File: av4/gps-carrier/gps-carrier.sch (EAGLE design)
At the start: 2 parts

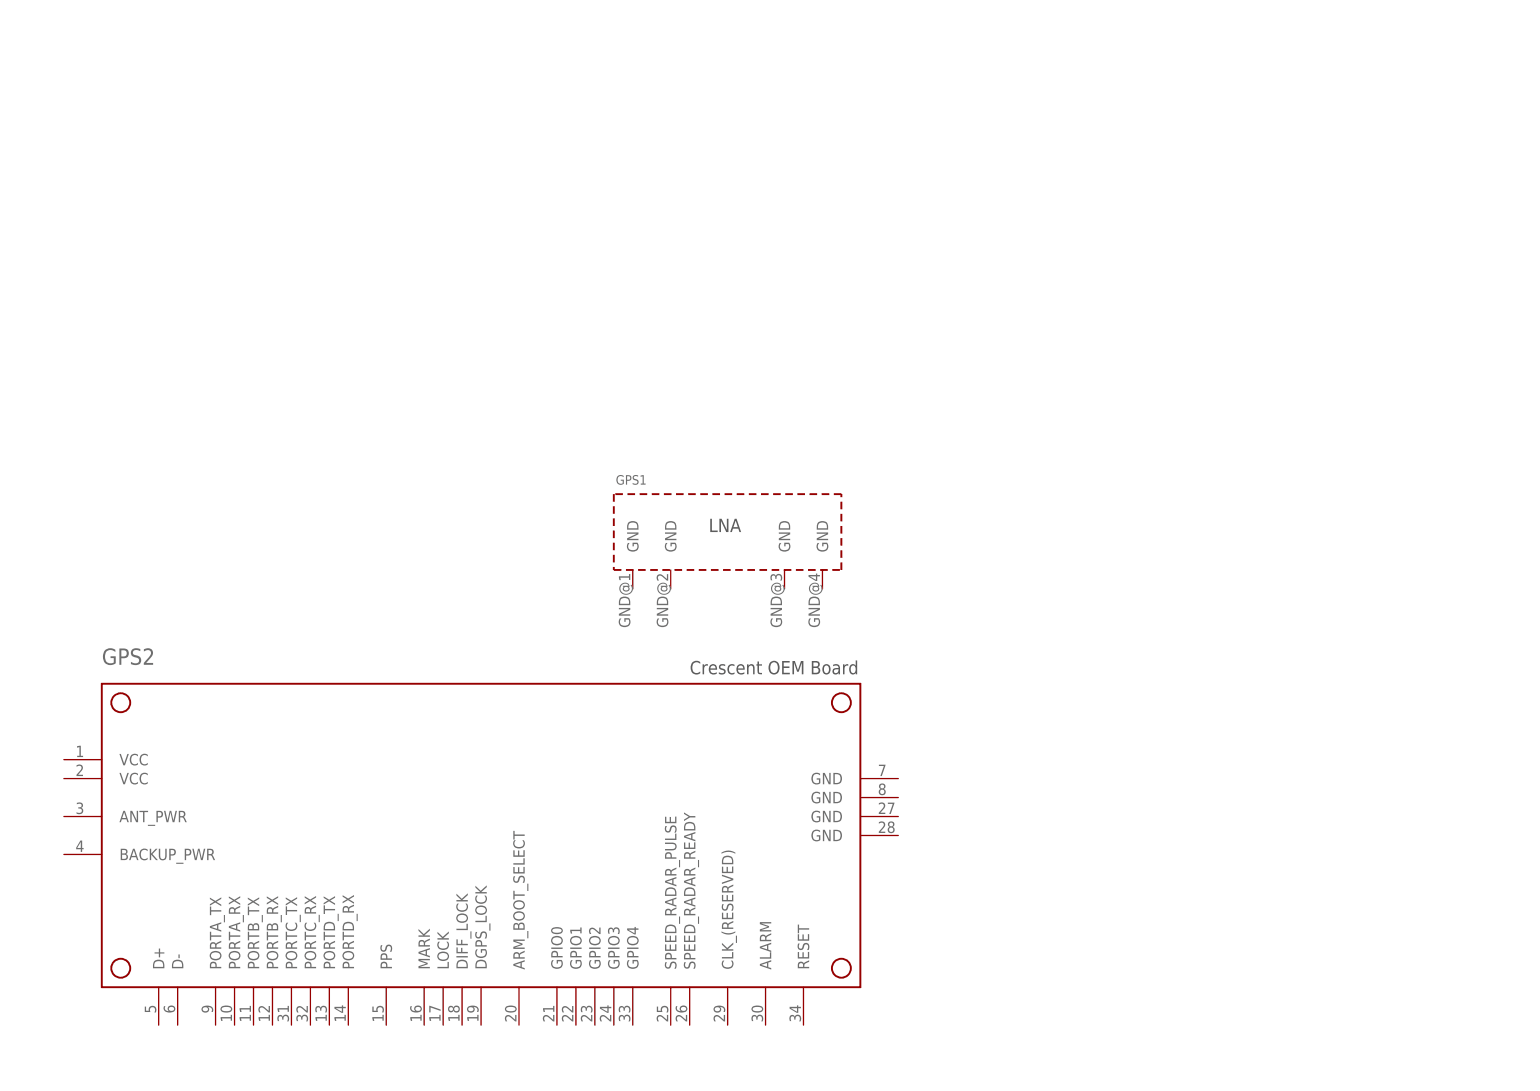
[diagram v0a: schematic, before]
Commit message: add headers
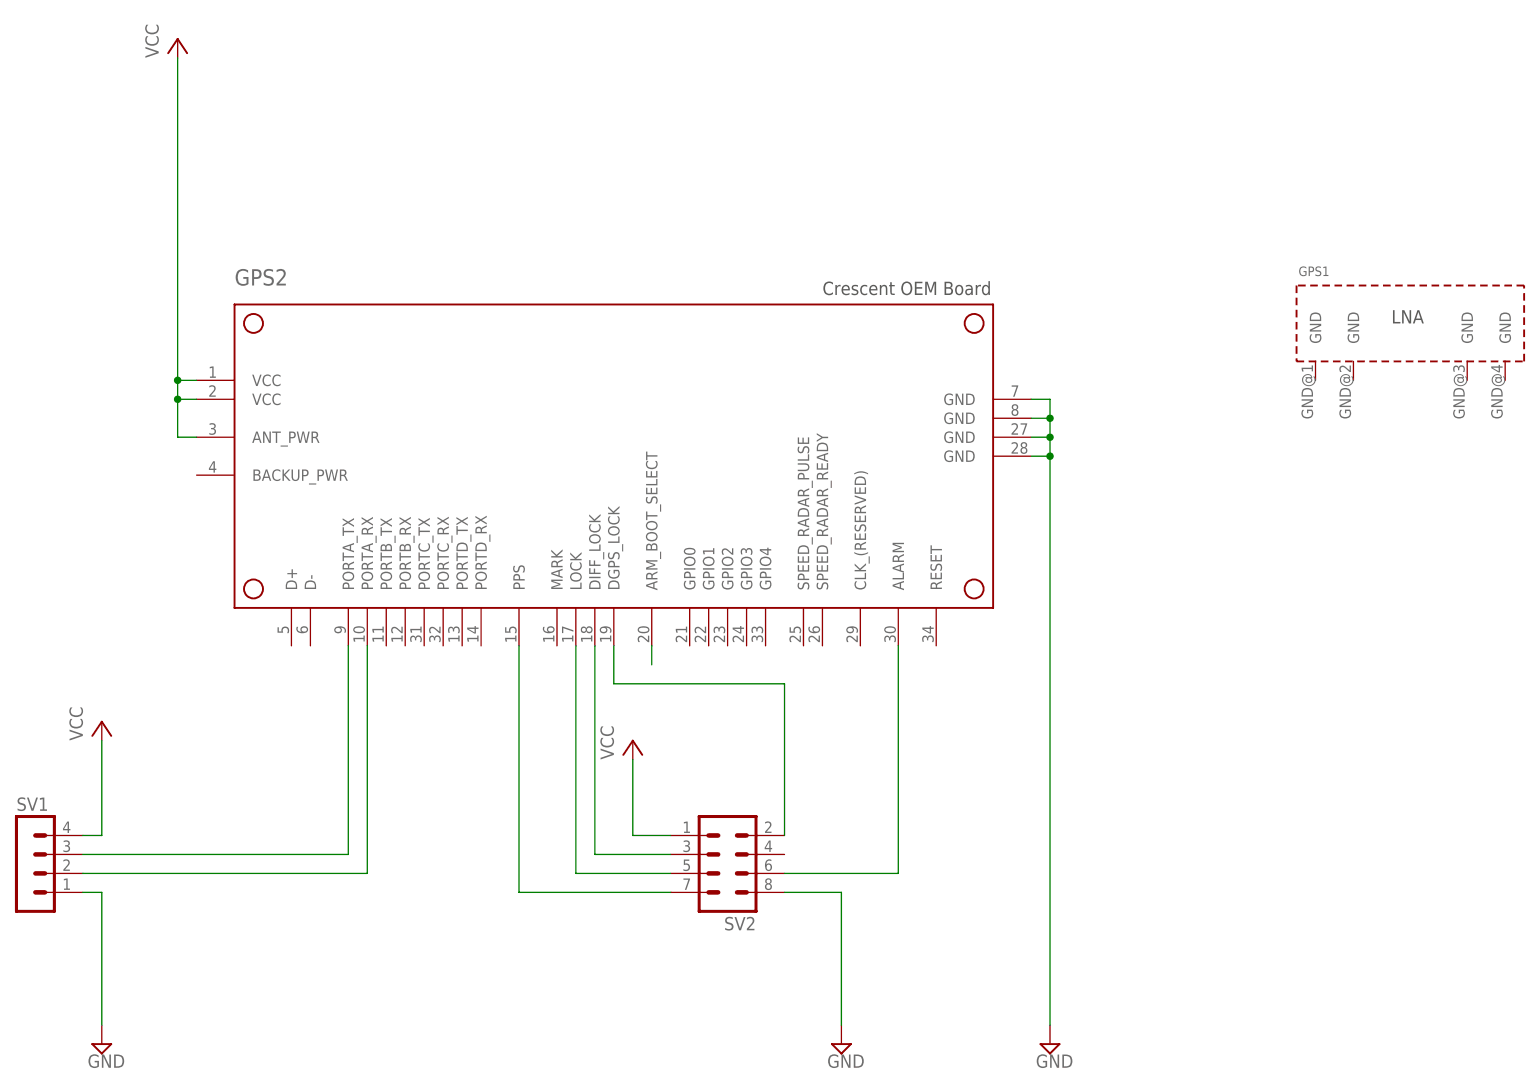
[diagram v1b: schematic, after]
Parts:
- added SV1: (no value), con-lstb:MA04-1
- added SV2: (no value), con-lstb:MA04-2
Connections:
- new net GND: GPS2.GND@1, GPS2.GND@2, GPS2.GND@3, GPS2.GND@4, SV1.1, SV2.8
- new net N$1: GPS2.PORTA_TX, SV1.3
- new net N$2: GPS2.PORTA_RX, SV1.2
- new net N$3: GPS2.PPS, SV2.7
- new net N$4: GPS2.LOCK, SV2.5
- new net N$5: GPS2.DIFF_LOCK, SV2.3
- new net N$6: GPS2.DGPS_LOCK, SV2.2
- new net N$8: GPS2.ALARM, SV2.6
- new net N$9: GPS2.ARM_BOOT_SELECT
- new net VCC: GPS2.ANT_PWR, GPS2.VCC@1, GPS2.VCC@2, SV1.4, SV2.1
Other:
- moved on the sheet: GPS1, GPS2
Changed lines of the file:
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@@
 <part name="GPS1" library="GPS_Hemisphere" deviceset="GPS_LNA" device=""/>
 <part name="GPS2" library="GPS_Hemisphere" deviceset="HEMISPHERE_GPS_MOUNT" device=""/>
+<part name="P+1" library="supply1" deviceset="VCC" device=""/>
+<part name="SUPPLY1" library="supply2" deviceset="GND" device=""/>
+<part name="SUPPLY2" library="supply2" deviceset="GND" device=""/>
+<part name="P+2" library="supply1" deviceset="VCC" device=""/>
+<part name="SV1" library="con-lstb" deviceset="MA04-1" device=""/>
+<part name="SV2" library="con-lstb" deviceset="MA04-2" device=""/>
+<part name="P+3" library="supply1" deviceset="VCC" device=""/>
+<part name="SUPPLY3" library="supply2" deviceset="GND" device=""/>
 </parts>
 <sheets>
@@
 </plain>
 <instances>
-<instance part="GPS1" gate="G$1" x="101.6" y="71.12"/>
-<instance part="GPS2" gate="G$1" x="68.58" y="30.48"/>
+<instance part="GPS1" gate="G$1" x="193.04" y="99.06"/>
+<instance part="GPS2" gate="G$1" x="86.36" y="81.28"/>
+<instance part="P+1" gate="VCC" x="27.94" y="137.16"/>
+<instance part="SUPPLY1" gate="GND" x="144.78" y="2.54"/>
+<instance part="SUPPLY2" gate="GND" x="17.78" y="2.54"/>
+<instance part="P+2" gate="VCC" x="17.78" y="45.72"/>
+<instance part="SV1" gate="1" x="7.62" y="27.94"/>
+<instance part="SV2" gate="G$1" x="101.6" y="25.4" rot="R180"/>
+<instance part="P+3" gate="VCC" x="88.9" y="43.18"/>
+<instance part="SUPPLY3" gate="GND" x="116.84" y="2.54"/>
 </instances>
 <busses>
 </busses>
 <nets>
+<net name="VCC" class="0">
+<segment>
+<pinref part="GPS2" gate="G$1" pin="VCC@1"/>
+<pinref part="P+1" gate="VCC" pin="VCC"/>
+<wire x1="30.48" y1="91.44" x2="27.94" y2="91.44" width="0.1524" layer="91"/>
+<wire x1="27.94" y1="91.44" x2="27.94" y2="134.62" width="0.1524" layer="91"/>
+<pinref part="GPS2" gate="G$1" pin="VCC@2"/>
+<wire x1="30.48" y1="88.9" x2="27.94" y2="88.9" width="0.1524" layer="91"/>
+<wire x1="27.94" y1="88.9" x2="27.94" y2="91.44" width="0.1524" layer="91"/>
+<junction x="27.94" y="91.44"/>
+<pinref part="GPS2" gate="G$1" pin="ANT_PWR"/>
+<wire x1="30.48" y1="83.82" x2="27.94" y2="83.82" width="0.1524" layer="91"/>
+<wire x1="27.94" y1="83.82" x2="27.94" y2="88.9" width="0.1524" layer="91"/>
+<junction x="27.94" y="88.9"/>
+</segment>
+<segment>
+<pinref part="P+2" gate="VCC" pin="VCC"/>
+<wire x1="17.78" y1="43.18" x2="17.78" y2="30.48" width="0.1524" layer="91"/>
+<pinref part="SV1" gate="1" pin="4"/>
+<wire x1="15.24" y1="30.48" x2="17.78" y2="30.48" width="0.1524" layer="91"/>
+</segment>
+<segment>
+<pinref part="SV2" gate="G$1" pin="1"/>
+<pinref part="P+3" gate="VCC" pin="VCC"/>
+<wire x1="93.98" y1="30.48" x2="88.9" y2="30.48" width="0.1524" layer="91"/>
+<wire x1="88.9" y1="30.48" x2="88.9" y2="40.64" width="0.1524" layer="91"/>
+</segment>
+</net>
+<net name="GND" class="0">
+<segment>
+<pinref part="GPS2" gate="G$1" pin="GND@4"/>
+<wire x1="142.24" y1="81.28" x2="144.78" y2="81.28" width="0.1524" layer="91"/>
+<pinref part="SUPPLY1" gate="GND" pin="GND"/>
+<wire x1="144.78" y1="81.28" x2="144.78" y2="5.08" width="0.1524" layer="91"/>
+<pinref part="GPS2" gate="G$1" pin="GND@3"/>
+<wire x1="142.24" y1="83.82" x2="144.78" y2="83.82" width="0.1524" layer="91"/>
+<wire x1="144.78" y1="83.82" x2="144.78" y2="81.28" width="0.1524" layer="91"/>
+<junction x="144.78" y="81.28"/>
+<junction x="144.78" y="83.82"/>
+<pinref part="GPS2" gate="G$1" pin="GND@1"/>
+<wire x1="142.24" y1="88.9" x2="144.78" y2="88.9" width="0.1524" layer="91"/>
+<wire x1="144.78" y1="88.9" x2="144.78" y2="86.36" width="0.1524" layer="91"/>
+<pinref part="GPS2" gate="G$1" pin="GND@2"/>
+<wire x1="144.78" y1="86.36" x2="144.78" y2="83.82" width="0.1524" layer="91"/>
+<wire x1="142.24" y1="86.36" x2="144.78" y2="86.36" width="0.1524" layer="91"/>
+<junction x="144.78" y="86.36"/>
+</segment>
+<segment>
+<pinref part="SUPPLY2" gate="GND" pin="GND"/>
+<wire x1="17.78" y1="5.08" x2="17.78" y2="22.86" width="0.1524" layer="91"/>
+<pinref part="SV1" gate="1" pin="1"/>
+<wire x1="15.24" y1="22.86" x2="17.78" y2="22.86" width="0.1524" layer="91"/>
+</segment>
+<segment>
+<pinref part="SV2" gate="G$1" pin="8"/>
+<pinref part="SUPPLY3" gate="GND" pin="GND"/>
+<wire x1="109.22" y1="22.86" x2="116.84" y2="22.86" width="0.1524" layer="91"/>
+<wire x1="116.84" y1="22.86" x2="116.84" y2="5.08" width="0.1524" layer="91"/>
+</segment>
+</net>
+<net name="N$1" class="0">
+<segment>
+<pinref part="GPS2" gate="G$1" pin="PORTA_TX"/>
+<wire x1="50.8" y1="55.88" x2="50.8" y2="27.94" width="0.1524" layer="91"/>
+<wire x1="50.8" y1="27.94" x2="15.24" y2="27.94" width="0.1524" layer="91"/>
+<pinref part="SV1" gate="1" pin="3"/>
+</segment>
+</net>
+<net name="N$2" class="0">
+<segment>
+<pinref part="GPS2" gate="G$1" pin="PORTA_RX"/>
+<wire x1="53.34" y1="55.88" x2="53.34" y2="25.4" width="0.1524" layer="91"/>
+<wire x1="53.34" y1="25.4" x2="15.24" y2="25.4" width="0.1524" layer="91"/>
+<pinref part="SV1" gate="1" pin="2"/>
+</segment>
+</net>
+<net name="N$3" class="0">
+<segment>
+<pinref part="SV2" gate="G$1" pin="7"/>
+<pinref part="GPS2" gate="G$1" pin="PPS"/>
+<wire x1="93.98" y1="22.86" x2="73.66" y2="22.86" width="0.1524" layer="91"/>
+<wire x1="73.66" y1="22.86" x2="73.66" y2="55.88" width="0.1524" layer="91"/>
+</segment>
+</net>
+<net name="N$4" class="0">
+<segment>
+<pinref part="SV2" gate="G$1" pin="5"/>
+<pinref part="GPS2" gate="G$1" pin="LOCK"/>
+<wire x1="93.98" y1="25.4" x2="81.28" y2="25.4" width="0.1524" layer="91"/>
+<wire x1="81.28" y1="25.4" x2="81.28" y2="55.88" width="0.1524" layer="91"/>
+</segment>
+</net>
+<net name="N$5" class="0">
+<segment>
+<pinref part="GPS2" gate="G$1" pin="DIFF_LOCK"/>
+<wire x1="83.82" y1="55.88" x2="83.82" y2="27.94" width="0.1524" layer="91"/>
+<pinref part="SV2" gate="G$1" pin="3"/>
+<wire x1="83.82" y1="27.94" x2="93.98" y2="27.94" width="0.1524" layer="91"/>
+</segment>
+</net>
+<net name="N$6" class="0">
+<segment>
+<pinref part="GPS2" gate="G$1" pin="DGPS_LOCK"/>
+<wire x1="86.36" y1="55.88" x2="86.36" y2="50.8" width="0.1524" layer="91"/>
+<pinref part="SV2" gate="G$1" pin="2"/>
+<wire x1="86.36" y1="50.8" x2="109.22" y2="50.8" width="0.1524" layer="91"/>
+<wire x1="109.22" y1="50.8" x2="109.22" y2="30.48" width="0.1524" layer="91"/>
+</segment>
+</net>
+<net name="N$8" class="0">
+<segment>
+<pinref part="GPS2" gate="G$1" pin="ALARM"/>
+<wire x1="124.46" y1="55.88" x2="124.46" y2="25.4" width="0.1524" layer="91"/>
+<pinref part="SV2" gate="G$1" pin="6"/>
+<wire x1="124.46" y1="25.4" x2="109.22" y2="25.4" width="0.1524" layer="91"/>
+</segment>
+</net>
+<net name="N$9" class="0">
+<segment>
+<pinref part="GPS2" gate="G$1" pin="ARM_BOOT_SELECT"/>
+<wire x1="91.44" y1="55.88" x2="91.44" y2="53.34" width="0.1524" layer="91"/>
+</segment>
+</net>
 </nets>
 </sheet>
